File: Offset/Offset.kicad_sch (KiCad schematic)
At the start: 51 parts, among them J1 Conn_02x05_Odd_Even, J10 AudioJack2_SwitchT, J11 AudioJack2_SwitchT, J12 AudioJack2_SwitchT, J13 AudioJack2_SwitchT, J2 AudioJack2_SwitchT, J3 AudioJack2_SwitchT, J4 AudioJack2_SwitchT, J5 AudioJack2_SwitchT, J6 AudioJack2_SwitchT, J7 AudioJack2_SwitchT, J8 AudioJack2_SwitchT, J9 AudioJack2_SwitchT, U1 TL072, U2 TL072, U3 TL072, U4 TL072, U5 TL072, U6 TL072

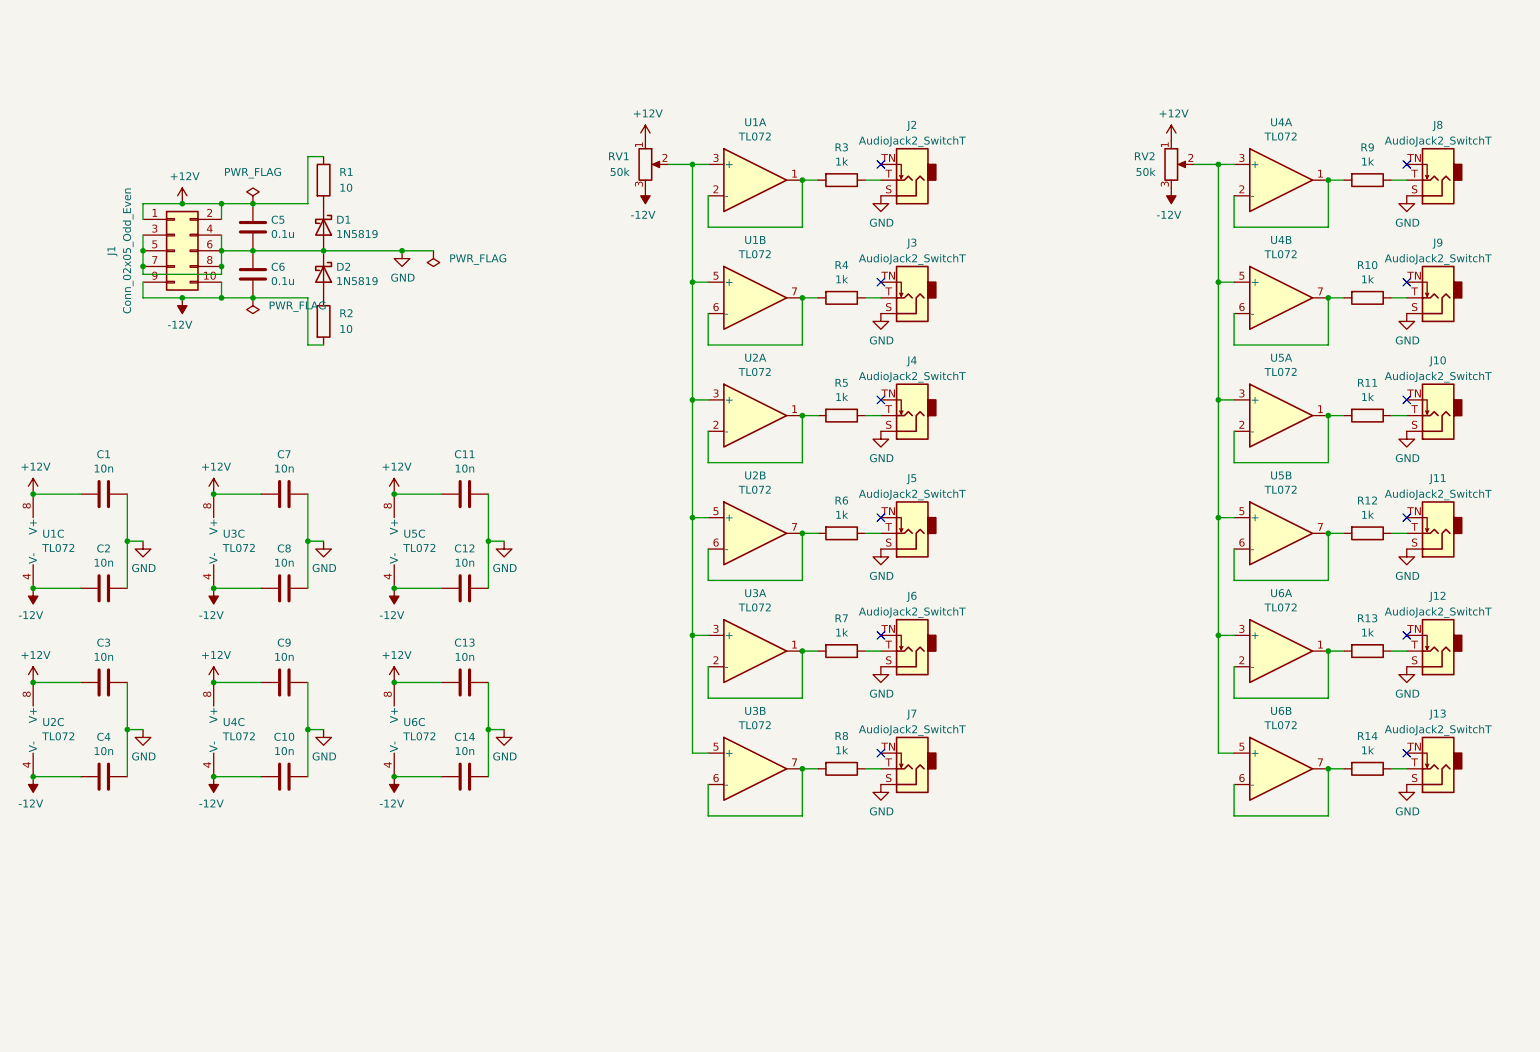
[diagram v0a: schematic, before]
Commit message: Begin revised delay
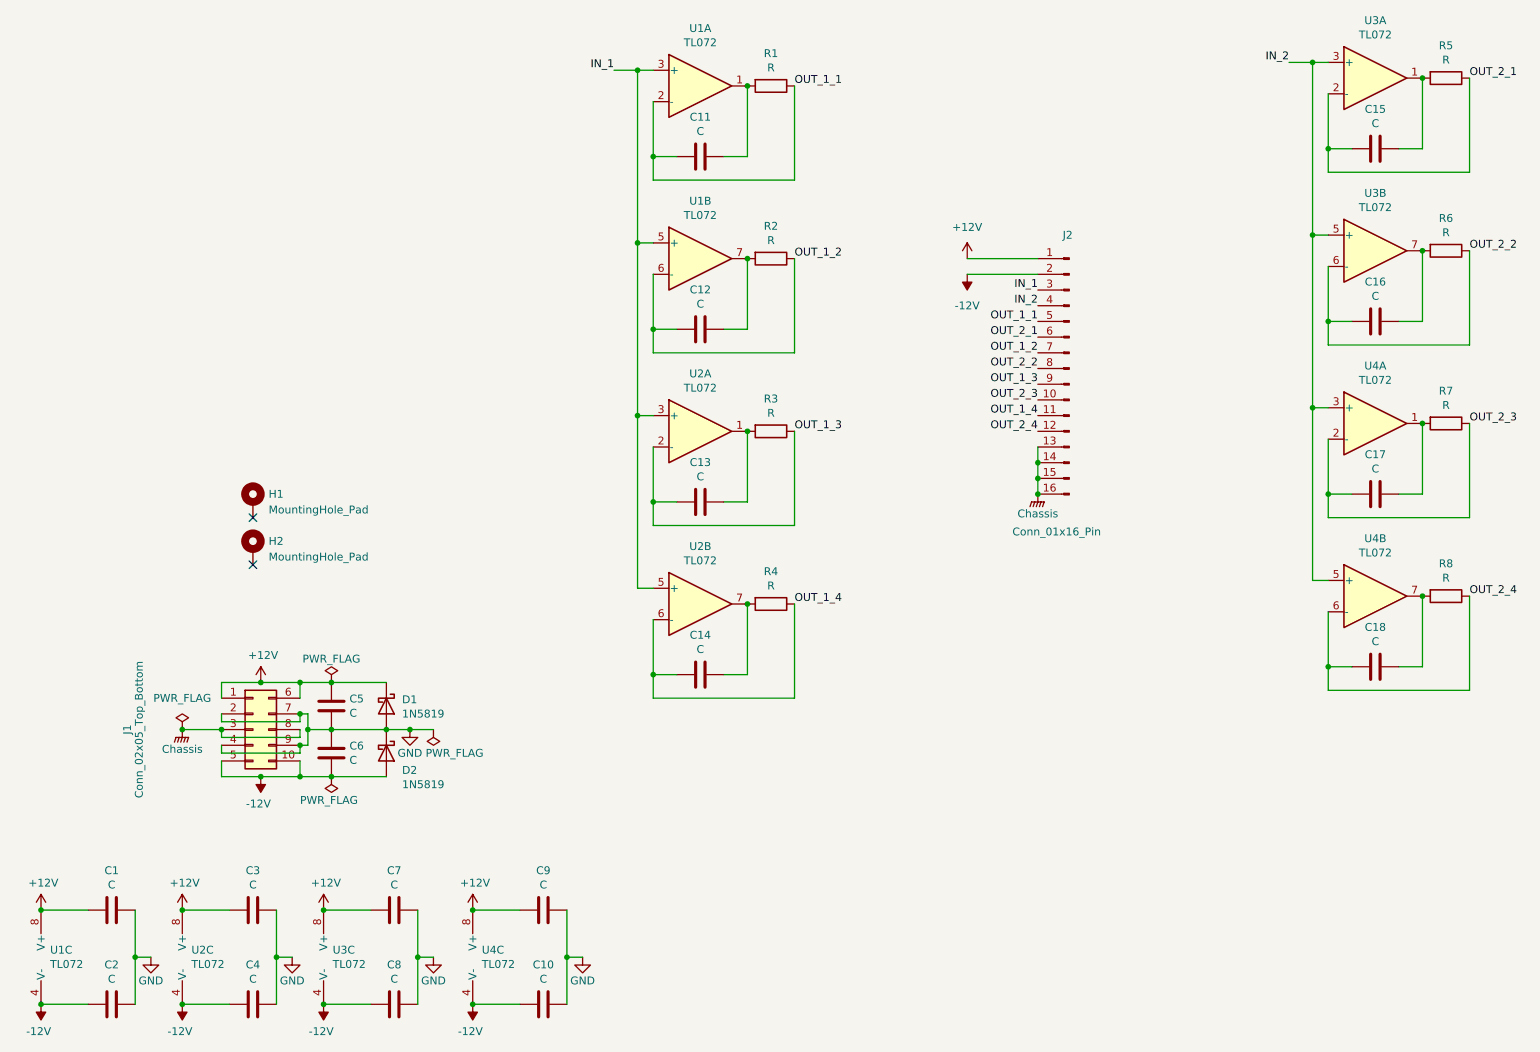
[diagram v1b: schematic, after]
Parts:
- removed J1: Conn_02x05_Odd_Even, Connector_PinHeader_2.54mm:PinHeader_2x05_P2.54mm_Vertical, symbol Connector_Generic:Conn_02x05_Odd_Even
- removed J10, J11, J12, J13, J2, J3, J4, J5, J6, J7, J8, J9: AudioJack2_SwitchT, Connector_Audio:Jack_3.5mm_QingPu_WQP-PJ398SM_Vertical_CircularHoles, symbol Connector:AudioJack2_SwitchT
- removed R10, R11, R12, R13, R14, R9: 1k, Resistor_THT:R_Axial_DIN0207_L6.3mm_D2.5mm_P7.62mm_Horizontal, symbol Device:R
- removed RV1, RV2: 50k, Potentiometer_THT:Potentiometer_Alpha_RD901F-40-00D_Single_Vertical_CircularHoles, symbol Device:R_Potentiometer
- removed U5, U6: TL072, Package_DIP:DIP-8_W7.62mm_Socket, symbol Amplifier_Operational:TL072
- added C15, C16, C17, C18: C, 0_Capacitor_THT:C_Disc_D5.5mm_W2.5mm_P2.50mm, symbol Device:C
- added H1, H2: MountingHole_Pad, 0_MountingHole:MountingHole_Pitch7.5mm_Drill3.4mm, symbol Mechanical:MountingHole_Pad
- added J1: Conn_02x05_Top_Bottom, Connector_Molex:Molex_Mini-Fit_Jr_5566-10A_2x05_P4.20mm_Vertical, symbol Connector_Generic:Conn_02x05_Top_Bottom
- added J2: Conn_01x16_Pin, Connector_PinHeader_2.54mm:PinHeader_1x16_P2.54mm_Vertical, symbol Connector:Conn_01x16_Pin
- C1, C10, C11, C12, C13, C14, C2, C3, C4, C7, C8, C9: value 10n -> C; footprint Capacitor_THT:C_Disc_D5.0mm_W2.5mm_P5.00mm -> 0_Capacitor_THT:C_Disc_D5.5mm_W2.5mm_P2.50mm
- C5, C6: value 0.1u -> C; footprint Capacitor_THT:C_Disc_D5.0mm_W2.5mm_P5.00mm -> 0_Capacitor_THT:C_Disc_D5.5mm_W4.0mm_P2.50mm
- R1, R2: value 10 -> R
- R3, R4, R5, R6, R7, R8: value 1k -> R
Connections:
- net +12V: now also D1.1 (K), J1.1 (Pin_1), J1.6 (Pin_6), J2.1 (Pin_1); no longer C11.1, C13.1, R1.1
- net -12V: now also D2.2 (A), J1.10 (Pin_10), J1.5 (Pin_5), J2.2 (Pin_2); no longer C12.1, C14.1, R2.2
- net GND: now also J1.2 (Pin_2), J1.4 (Pin_4), J1.7 (Pin_7), J1.9 (Pin_9); no longer C11.2, C12.2, C13.2, C14.2
- net at U4.7: now also R8.2, C18.2; no longer U4.6 (-)
- net OUT_2_2: now reaches R6.1
- net OUT_2_2: now also U3.6 (-), C16.1, J2.8 (Pin_8)
- net IN_2: now reaches U4.3 (+), U4.5 (+)
- net IN_2: now also U3.3 (+), U3.5 (+), J2.4 (Pin_4)
- net OUT_1_2: now reaches R2.1
- net OUT_1_2: now also C12.1, U1.6 (-), J2.7 (Pin_7); no longer D2.2 (A)
- net OUT_1_3: now reaches R3.1
- net OUT_1_3: now also C13.1, U2.2 (-), J2.9 (Pin_9)
- net at R1.2: now also C11.2, U1.1; no longer D1.1 (K)
- net OUT_2_4: now reaches R8.1
- net OUT_2_4: now also U4.6 (-), C18.1, J2.12 (Pin_12)
- net IN_1: now reaches U1.3 (+), U1.5 (+), U2.3 (+), U2.5 (+)
- net IN_1: now also J2.3 (Pin_3); no longer U3.3 (+), U3.5 (+)
- net OUT_2_1: now reaches R5.1
- net OUT_2_1: now also U3.2 (-), C15.1, J2.6 (Pin_6)
- net at U4.1: now also R7.2, C17.2; no longer U4.2 (-)
- net OUT_2_3: now reaches R7.1
- net OUT_2_3: now also U4.2 (-), C17.1, J2.10 (Pin_10)
- net OUT_1_4: now reaches R4.1
- net OUT_1_4: now also C14.1, U2.6 (-), J2.11 (Pin_11)
- new net: C13.2, R3.2, U2.1
- new net: C15.2, R5.2, U3.1
- new net: C14.2, R4.2, U2.7
- new net: C12.2, R2.2, U1.7
- new net: C16.2, R6.2, U3.7
- new net Chassis: J1.3 (Pin_3), J1.8 (Pin_8), J2.13 (Pin_13), J2.14 (Pin_14), J2.15 (Pin_15), J2.16 (Pin_16)
- new net OUT_1_1: C11.1, J2.5 (Pin_5), R1.1, U1.2 (-)
- no-connect marks 12 -> 2
